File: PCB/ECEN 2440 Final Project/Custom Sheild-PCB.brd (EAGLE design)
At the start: 63.2 x 102.9 mm, 10 parts

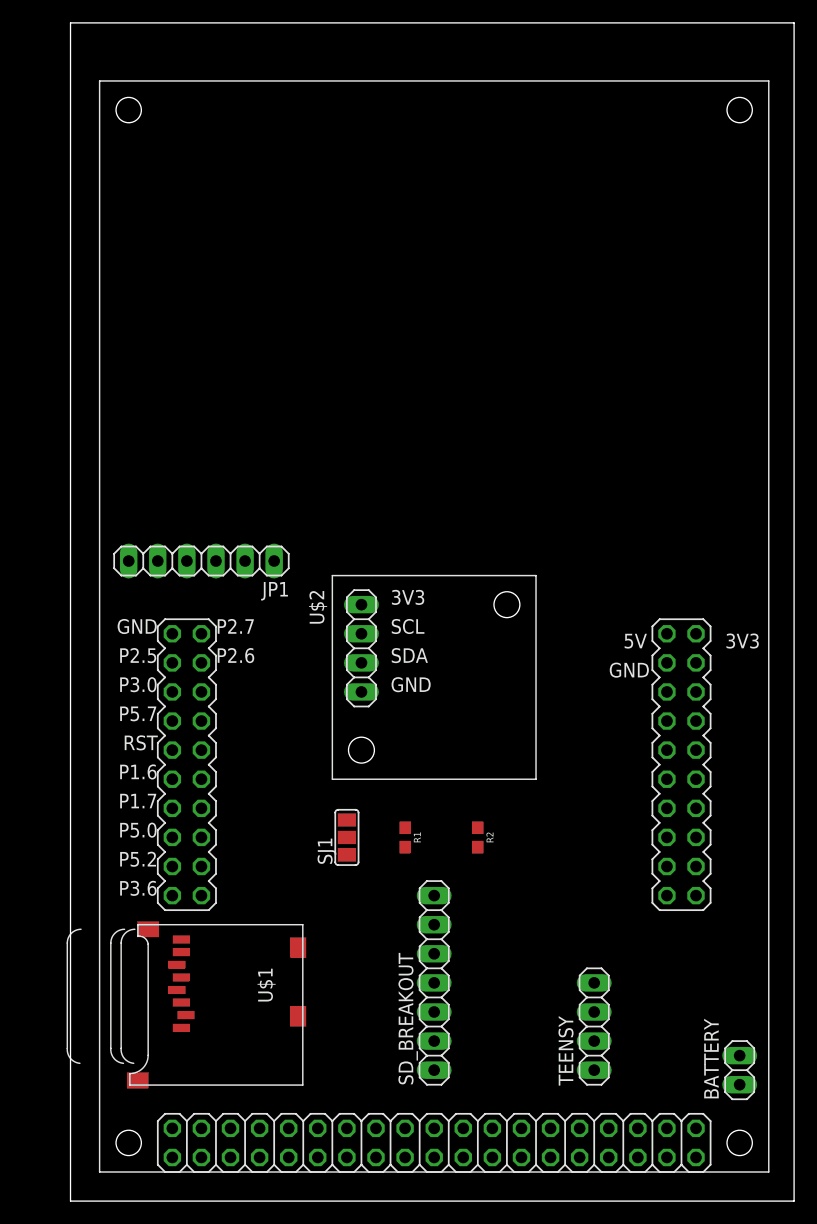
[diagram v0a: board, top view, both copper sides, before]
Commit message: prettyfy schematic. vague shield board layout.
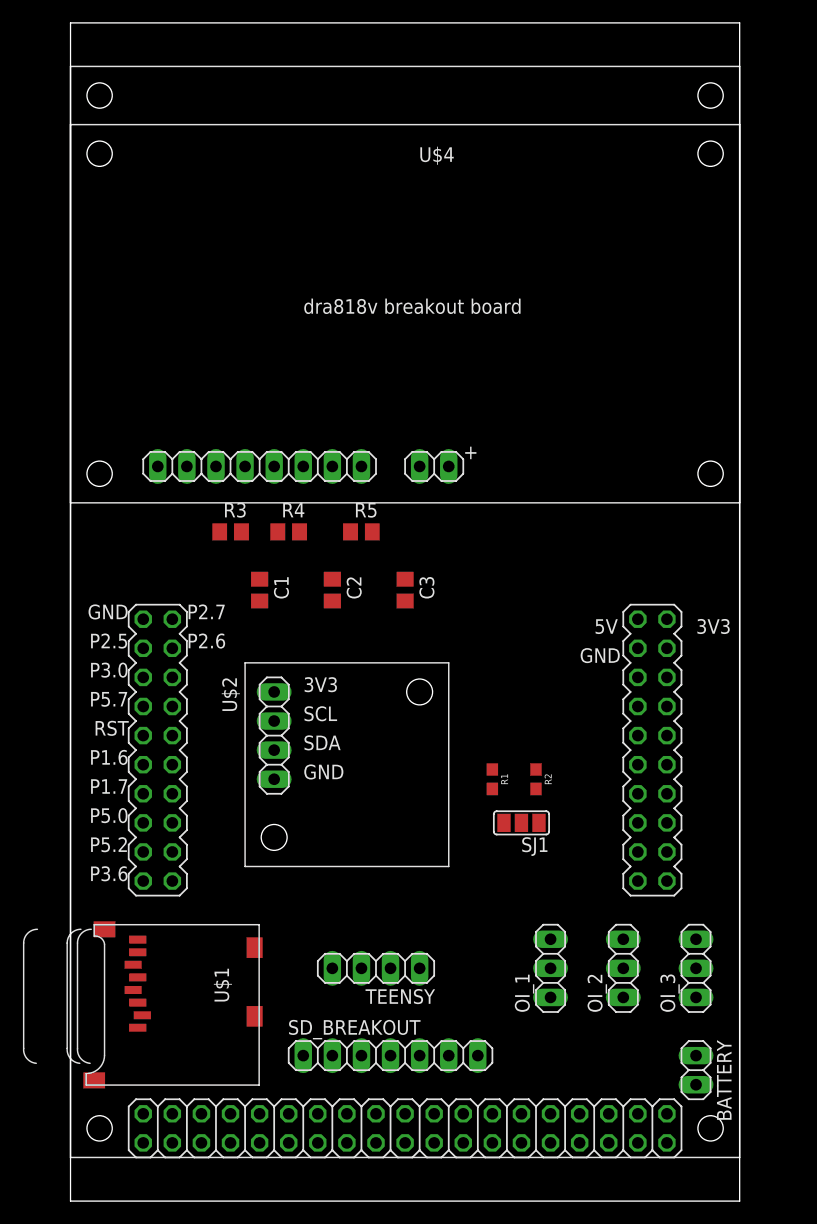
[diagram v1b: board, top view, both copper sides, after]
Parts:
- removed JP1: (no value), pinhead:1X06
- added C1, C2, C3: 500n, rcl:C0805
- added OI_1, OI_2, OI_3: (no value), pinhead:1X03
- added R3, R4, R5: 100R, rcl:R0805
- added U$4: DRA_BREAKOUT, Custom Library:DRA_BREAKOUT
- moved TEENSY 19.7 mm to (26.7, 20.3), turned to 180 degrees
- moved SJ1 15.3 mm to (39.4, 33.0), turned to 180 degrees
- moved U$2 10.8 mm to (15.2, 29.2)
- moved R1 9.16 mm to (36.8, 36.8)
- moved SD_BREAKOUT 7.41 mm to (27.9, 12.7), turned to 0 degrees
- moved R2 7.18 mm to (40.6, 36.8)
- moved BATTERY 3.81 mm to (54.6, 11.4), turned to 270 degrees
- moved U$1 3.81 mm to (16.5, 24.1)
- moved U$3 2.84 mm to (0.00, 3.81)
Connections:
- net CD1 renamed SD_CD1
- new net AUDIO_FILTERED: C3.1, R5.2, U$4.MIC_IN
- new net N$3: C1.1, R3.2, R4.1
- new net N$4: C2.1, R4.2, R5.1
- new net OI_1: OI_1.2, U$3.9.1
- new net OI_2: OI_2.2, U$3.9.2
- new net OI_3: OI_3.2, U$3.9.3
- new net PD_RADIO: U$4.PD
- new net RADIO_PD: U$3.P4.1
- net +3V3: now also OI_1.3, OI_2.3, OI_3.3; no longer JP1.6
- net AUDIO_PTT: now also U$4.PTT; no longer JP1.4
- net AUDIO_PWM: now also R3.1; no longer JP1.3
- net GND: now also C1.2, C2.2, C3.2, OI_1.1, OI_2.1, OI_3.1, U$4.GND; no longer JP1.5
- net RX_RADIO: now also U$4.RX_RADIO; no longer JP1.2
- net TX_RADIO: now also U$4.TX_RADIO; no longer JP1.1
- net VCC: now also U$4.VCC
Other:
- board size 63.2 x 102.9 mm -> 58.4 x 102.9 mm
